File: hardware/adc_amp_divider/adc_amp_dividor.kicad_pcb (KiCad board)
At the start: 2 copper layers, 76.2 x 52.7 mm, 118 parts, among them M1 CONN_1, M2 CONN_1, M3 CONN_1, P1 CONN_10X2, P2 CONN_6, P3 CONN_6, P4 CONN_3, P5 CONN_2, P6 CONN_1, P7 CONN_1, P8 CONN_3, P9 CONN_2, U1 LMV324IDR, U2 LMV324IDR, U3 LMV324IDR

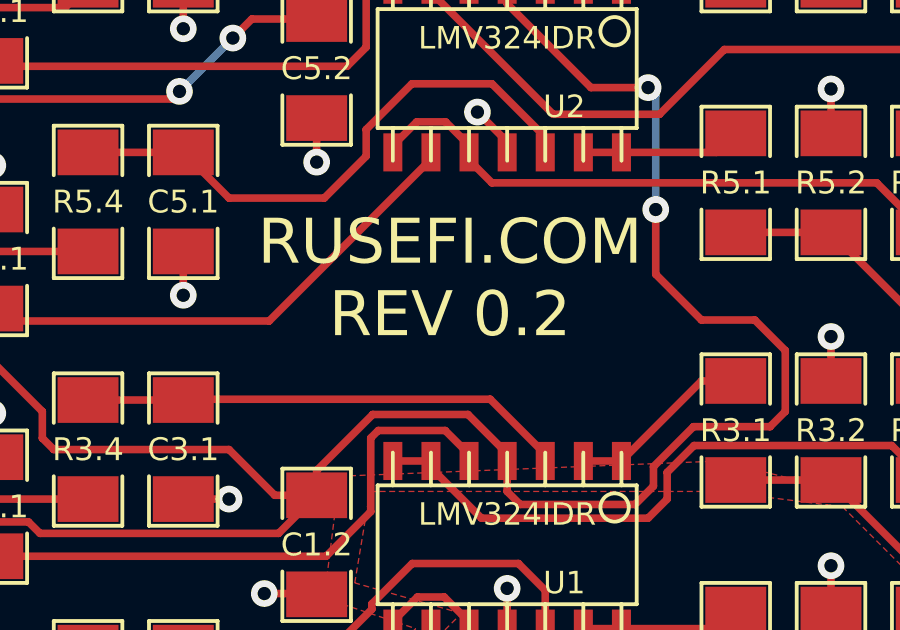
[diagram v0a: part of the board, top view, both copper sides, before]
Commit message: silkscreen
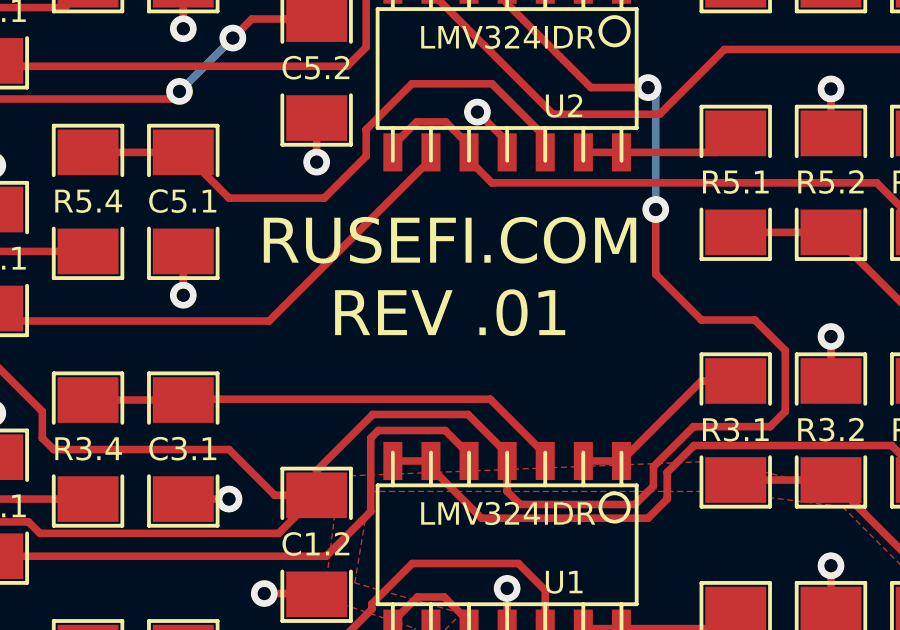
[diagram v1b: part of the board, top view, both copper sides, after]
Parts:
- R1, R1.4, R10.4, R11.4, R12.4, R2.4, R3.4, R4.4, R5.4, R6.4, R7.4, R8.4, R9.4: value 100 -> 150
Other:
- board text added: "RUSEFI.COM REV .01"
- board text removed: "RUSEFI.COM REV 0.2"
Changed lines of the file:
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@@
     (links 234)
     (no_connects 0)
-    (area 76.455001 116.9924 170.180001 180.5)
+    (area 68.835001 116.9924 170.180001 180.5)
     (thickness 1.6)
-    (drawings 9)
+    (drawings 10)
     (tracks 802)
     (zones 0)
@@
     (nets 68)
   )
-  (page A3)
+  (page A)
+  (title_block
+    (title "Analgo Protection board for RUSEFI.com")
+    (rev .01)
+    (company RUSEFI.com)
+  )
   (layers
     (15 F.Cu signal)
@@
       (effects (font (size 0.762 0.762) (thickness 0.127)))
     )
-    (fp_text value 100 (at 0 0 90) (layer F.SilkS) hide
+    (fp_text value 150 (at 0 0 90) (layer F.SilkS) hide
       (effects (font (size 0.762 0.762) (thickness 0.127)))
     )
@@
       (effects (font (size 0.762 0.762) (thickness 0.127)))
     )
-    (fp_text value 100 (at 0 0 270) (layer F.SilkS) hide
+    (fp_text value 150 (at 0 0 270) (layer F.SilkS) hide
       (effects (font (size 0.762 0.762) (thickness 0.127)))
     )
@@
       (effects (font (size 0.762 0.762) (thickness 0.127)))
     )
-    (fp_text value 100 (at 0 0 90) (layer F.SilkS) hide
+    (fp_text value 150 (at 0 0 90) (layer F.SilkS) hide
       (effects (font (size 0.762 0.762) (thickness 0.127)))
     )
@@
       (effects (font (size 0.762 0.762) (thickness 0.127)))
     )
-    (fp_text value 100 (at 0 0 270) (layer F.SilkS) hide
+    (fp_text value 150 (at 0 0 270) (layer F.SilkS) hide
       (effects (font (size 0.762 0.762) (thickness 0.127)))
     )
@@
       (effects (font (size 0.762 0.762) (thickness 0.127)))
     )
-    (fp_text value 100 (at 0 0 270) (layer F.SilkS) hide
+    (fp_text value 150 (at 0 0 270) (layer F.SilkS) hide
       (effects (font (size 0.762 0.762) (thickness 0.127)))
     )
@@
       (effects (font (size 0.762 0.762) (thickness 0.127)))
     )
-    (fp_text value 100 (at 0 0 90) (layer F.SilkS) hide
+    (fp_text value 150 (at 0 0 90) (layer F.SilkS) hide
       (effects (font (size 0.762 0.762) (thickness 0.127)))
     )
@@
       (effects (font (size 0.762 0.762) (thickness 0.127)))
     )
-    (fp_text value 100 (at 0 0) (layer F.SilkS) hide
+    (fp_text value 150 (at 0 0) (layer F.SilkS) hide
       (effects (font (size 0.762 0.762) (thickness 0.127)))
     )
@@
       (effects (font (size 0.762 0.762) (thickness 0.127)))
     )
-    (fp_text value 100 (at 0 0 90) (layer F.SilkS) hide
+    (fp_text value 150 (at 0 0 90) (layer F.SilkS) hide
       (effects (font (size 0.762 0.762) (thickness 0.127)))
     )
@@
       (effects (font (size 0.762 0.762) (thickness 0.127)))
     )
-    (fp_text value 100 (at 0 0 270) (layer F.SilkS) hide
+    (fp_text value 150 (at 0 0 270) (layer F.SilkS) hide
       (effects (font (size 0.762 0.762) (thickness 0.127)))
     )
@@
       (effects (font (size 0.762 0.762) (thickness 0.127)))
     )
-    (fp_text value 100 (at 0 0 270) (layer F.SilkS) hide
+    (fp_text value 150 (at 0 0 270) (layer F.SilkS) hide
       (effects (font (size 0.762 0.762) (thickness 0.127)))
     )
@@
       (effects (font (size 0.762 0.762) (thickness 0.127)))
     )
-    (fp_text value 100 (at 0 0 90) (layer F.SilkS) hide
+    (fp_text value 150 (at 0 0 90) (layer F.SilkS) hide
       (effects (font (size 0.762 0.762) (thickness 0.127)))
     )
@@
       (effects (font (size 0.762 0.762) (thickness 0.127)))
     )
-    (fp_text value 100 (at 0 0 90) (layer F.SilkS) hide
+    (fp_text value 150 (at 0 0 90) (layer F.SilkS) hide
       (effects (font (size 0.762 0.762) (thickness 0.127)))
     )
@@
       (effects (font (size 0.762 0.762) (thickness 0.127)))
     )
-    (fp_text value 100 (at 0 0 270) (layer F.SilkS) hide
+    (fp_text value 150 (at 0 0 270) (layer F.SilkS) hide
       (effects (font (size 0.762 0.762) (thickness 0.127)))
     )
@@
     )
   )
-  (gr_text "RUSEFI.COM\nREV 0.2" (at 135.255 152.4) (layer F.SilkS)
+  (dimension 50.165 (width 0.3) (layer Dwgs.User)
+    (gr_text "50.165 mm" (at 75.485 147.0025 90) (layer Dwgs.User)
+      (effects (font (size 1.5 1.5) (thickness 0.3)))
+    )
+    (feature1 (pts (xy 80.01 121.92) (xy 74.135 121.92)))
+    (feature2 (pts (xy 80.01 172.085) (xy 74.135 172.085)))
+    (crossbar (pts (xy 76.835 172.085) (xy 76.835 121.92)))
+    (arrow1a (pts (xy 76.835 121.92) (xy 77.42142 123.046503)))
+    (arrow1b (pts (xy 76.835 121.92) (xy 76.24858 123.046503)))
+    (arrow2a (pts (xy 76.835 172.085) (xy 77.42142 170.958497)))
+    (arrow2b (pts (xy 76.835 172.085) (xy 76.24858 170.958497)))
+  )
+  (gr_text "RUSEFI.COM\nREV .01" (at 135.255 152.4) (layer F.SilkS)
     (effects (font (size 1.5 1.5) (thickness 0.3)))
   )
